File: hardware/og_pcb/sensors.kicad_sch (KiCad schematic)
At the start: 10 parts, among them U13 INA219AxD, U15 TMP1075DSG, U6 INA260

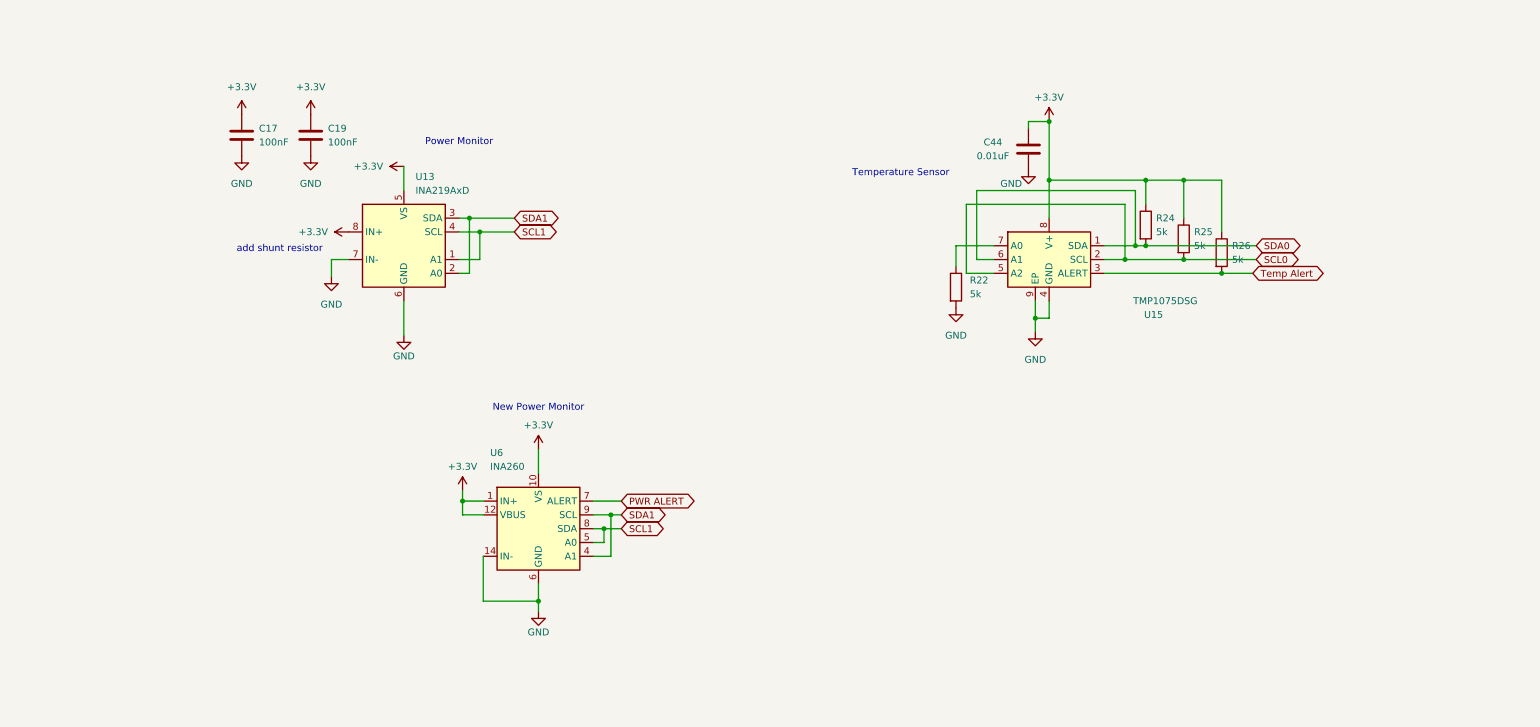
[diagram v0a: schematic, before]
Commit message: new preliminary demo pcb
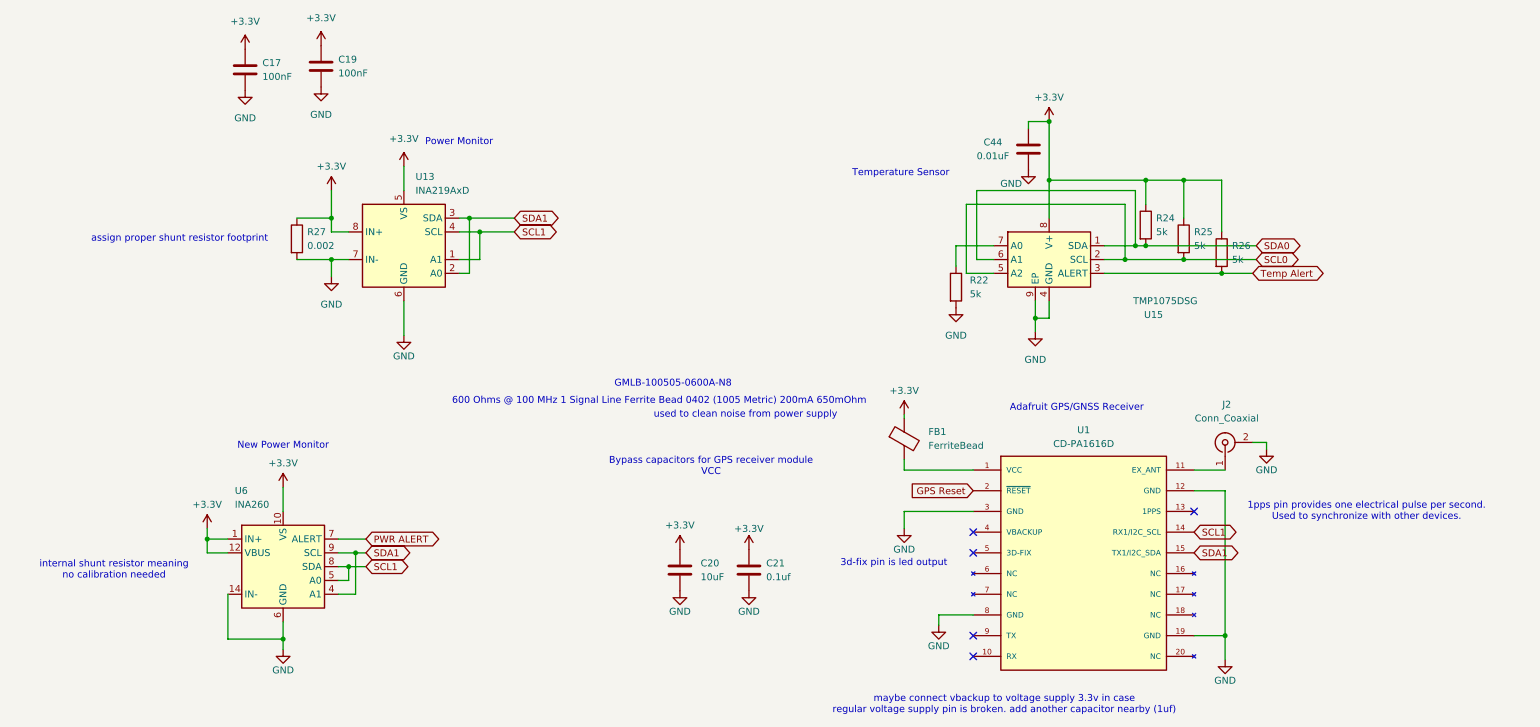
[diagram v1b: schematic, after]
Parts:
- added C20: 10uF, Capacitor_SMD:C_0402_1005Metric, symbol Device:C
- added C21: 0.1uf, Capacitor_SMD:C_0402_1005Metric, symbol Device:C
- added FB1: FerriteBead, symbol Device:FerriteBead
- added J2: Conn_Coaxial, Connector_Coaxial:MMCX_Molex_73415-1471_Vertical, symbol Connector:Conn_Coaxial
- added R27: 0.002, Resistor_SMD:R_0402_1005Metric, symbol Device:R
- added U1: CD-PA1616D, 1my_footprints:CD-PA1616D, symbol CD-PA1616D:CD-PA1616D
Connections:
- net +3.3V: now also C20.1, C21.1, FB1.1, R27.1
- net GND: now also C20.2, C21.2, J2.2 (Ext), R27.2, U1.12 (GND), U1.19 (GND), U1.3 (GND), U1.8 (GND)
- net SCL1: now also U1.14 (RX1/I2C_SCL)
- net SDA1: now also U1.15 (TX1/I2C_SDA)
- new net: J2.1 (In), U1.11 (EX_ANT)
- new net: FB1.2, U1.1 (VCC)
- new net GPS Reset: U1.2 (~{RESET})
- no-connect marks 0 -> 5
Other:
- note added: "1pps pin provides one electrical pulse per second. Used to synchronize with other devices."
- note added: "3d-fix pin is led output"
- note added: "600 Ohms @ 100 MHz 1 Signal Line Ferrite Bead 0402 (1005 Metric) 200mA 650mOhm"
- note added: "Adafruit GPS/GNSS Receiver"
- note added: "Bypass capacitors for GPS receiver module VCC"
- note added: "GMLB-100505-0600A-N8"
- note added: "assign proper shunt resistor footprint"
- note added: "internal shunt resistor meaning no calibration needed"
- note added: "maybe connect vbackup to voltage supply 3.3v in case regular voltage supply pin is broken. add another capacitor nearby (1uf)"
- note added: "used to clean noise from power supply"
- note removed: "add shunt resistor"
- moved on the sheet: C17, C19, U6
